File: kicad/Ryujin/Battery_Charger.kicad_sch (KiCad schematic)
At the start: 26 parts, among them Q3 Q1, Q4 Q2, U6 BQ24650

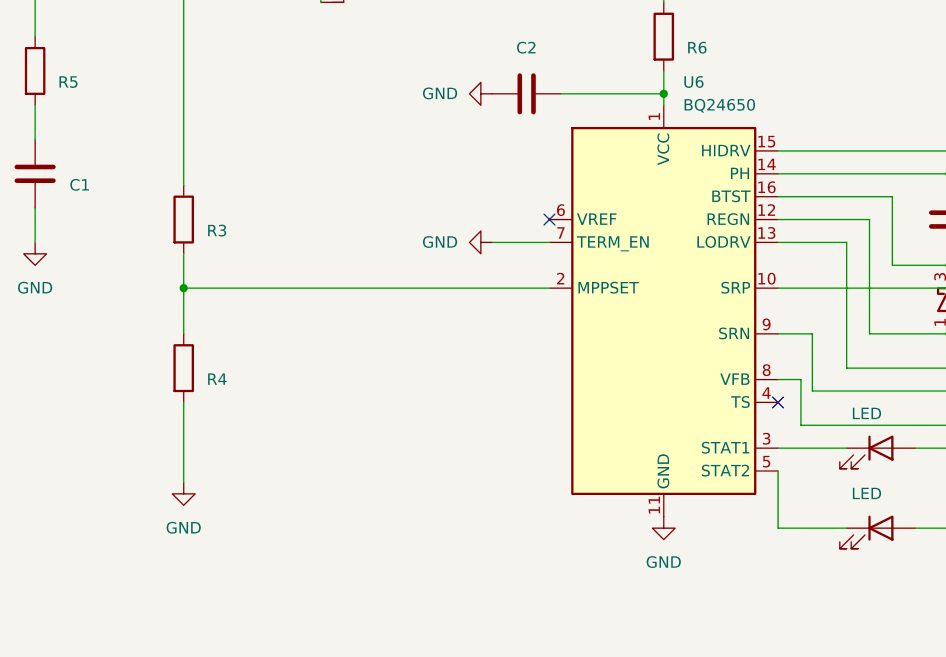
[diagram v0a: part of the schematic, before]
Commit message: Lost Mariner
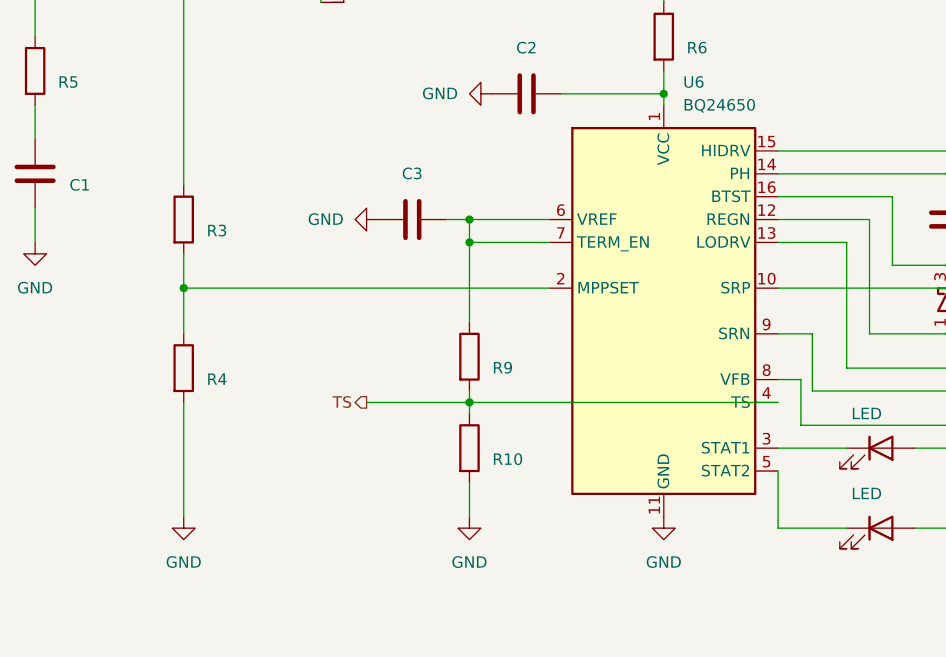
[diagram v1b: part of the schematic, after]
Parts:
- added C15: C3, Capacitor_SMD:C_0805_2012Metric, symbol Device:C
- added R14: R9, Resistor_SMD:R_0402_1005Metric, symbol Device:R
- added R17: R10, Resistor_SMD:R_0402_1005Metric, symbol Device:R
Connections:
- net GND: now also C15.1, R17.2; no longer U6.7 (TERM_EN)
- net TS: now reaches U6.4 (TS)
- net TS: now also R14.2, R17.1
- net at U6.6 (VREF): now also U6.7 (TERM_EN), C15.2, R14.1
- no-connect marks 2 -> 0
